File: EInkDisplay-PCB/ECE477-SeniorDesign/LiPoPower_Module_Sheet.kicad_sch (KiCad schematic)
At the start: 21 parts, among them J6 Battery Connector, U2 MCP73871, U4 TPS63060, U5 BQ27441-G1

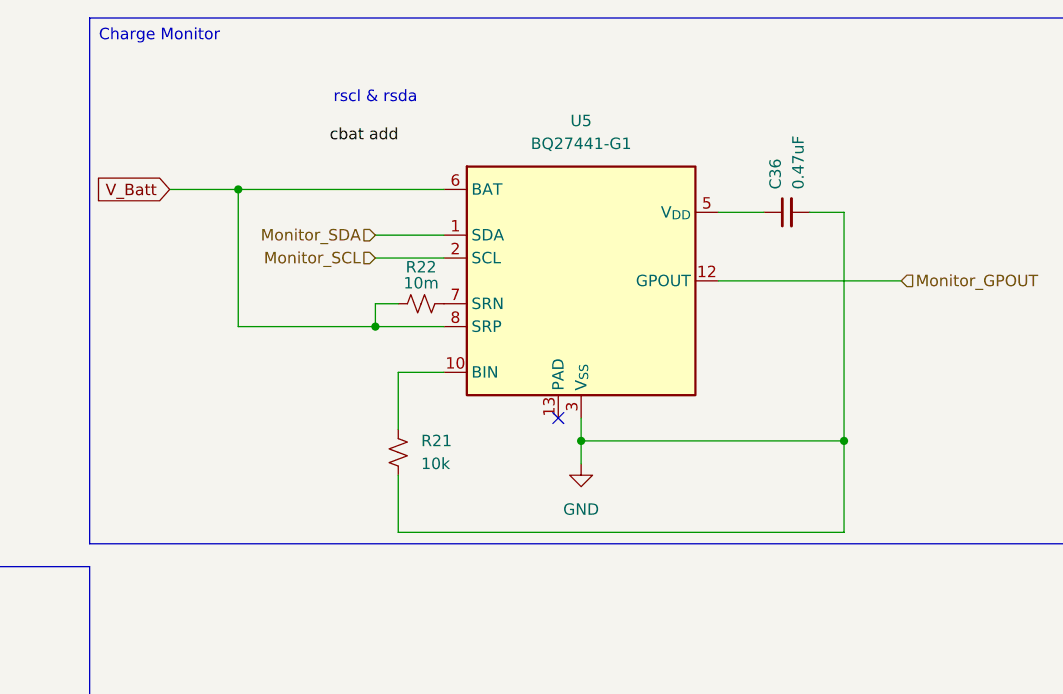
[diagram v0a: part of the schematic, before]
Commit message: Update LiPoPower_Module_Sheet.kicad_sch
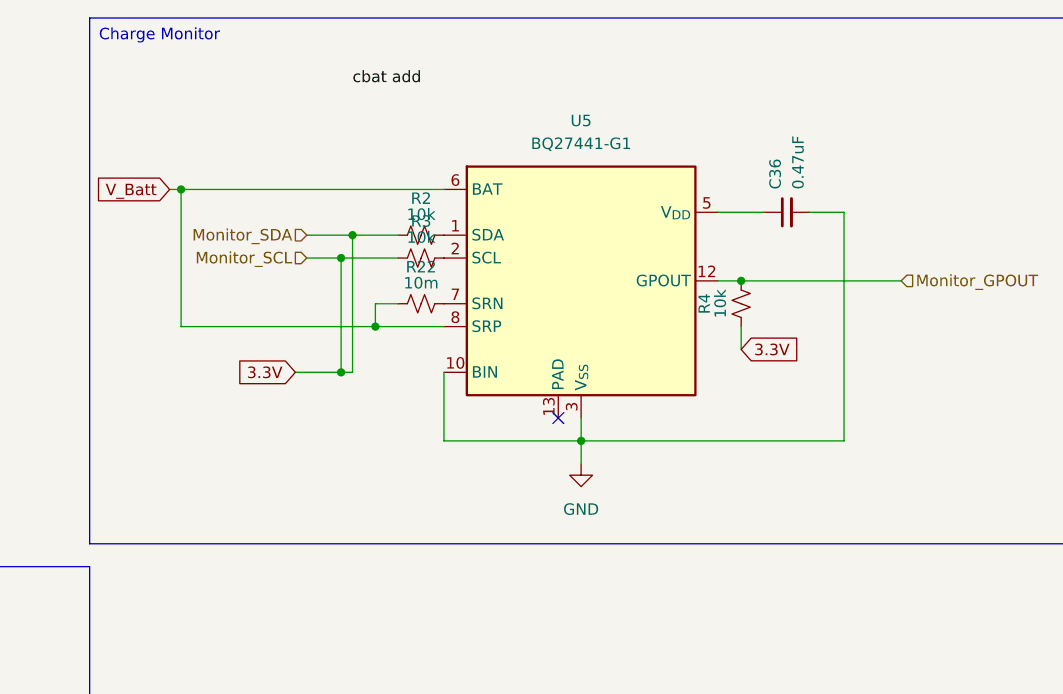
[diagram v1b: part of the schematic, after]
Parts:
- removed R21: 10k, Resistor_SMD:R_0805_2012Metric_Pad1.20x1.40mm_HandSolder, symbol Device:R_Small_US
- added R2, R3, R4: 10k, Resistor_SMD:R_0805_2012Metric_Pad1.20x1.40mm_HandSolder, symbol Device:R_Small_US
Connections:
- net GND: now also U5.10 (BIN)
- net Monitor_GPOUT: now also R4.2
- net Monitor_SCL: no longer names the net of U5.2 (SCL)
- net Monitor_SCL: now also R3.2
- net Monitor_SDA: no longer names the net of U5.1 (SDA)
- net Monitor_SDA: now also R2.2
- new net 3.3V: R2.1, R3.1, R4.1
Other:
- note removed: "rscl & rsda"
